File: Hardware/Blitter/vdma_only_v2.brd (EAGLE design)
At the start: 100 x 157.5 mm, 84 parts, among them IC1 74S08N, IC10 74HC191N, IC11 74HC191N, IC12 74HC191N, IC13 74HC191N, IC14 74HC191N, IC15 74HC191N, IC16 74HC573N, IC17 74HC573N, IC18 7432N, IC19 74LS257N, IC2 74HC191N, IC20 7430N, IC21 7400N, IC22 74LS257N, IC23 74LS257N, IC24 74LS257N, IC25 74LS257N, IC26 74LS257N, IC27 74LS257N, IC28 74LS257N, IC29 74LS257N, IC3 74HC573N, IC30 74HC573N, IC31 7400N, IC32 7432N, IC33 7400N, IC4 74HC191N, IC5 74HC573N, IC53 7404N, IC54 74LS07N, IC6 74HC573N, IC7 74HC573N, IC8 74HC573N, IC9 74LS74N, J1 TX25-40P-6ST-H1E, J2 TX25-40P-6ST-H1E

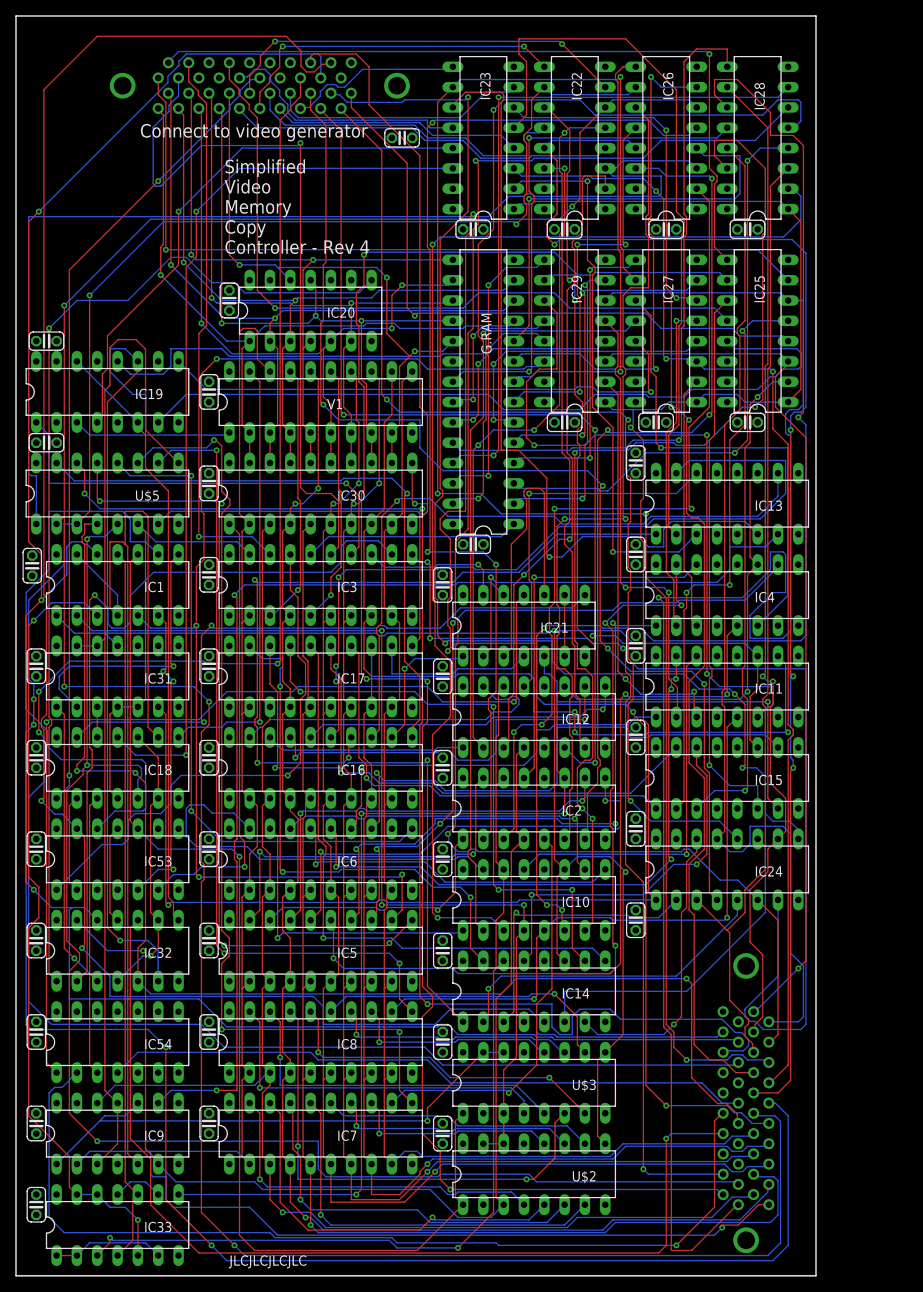
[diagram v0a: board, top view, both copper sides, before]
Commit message: regrettably I don't remember what I changed since the last commit
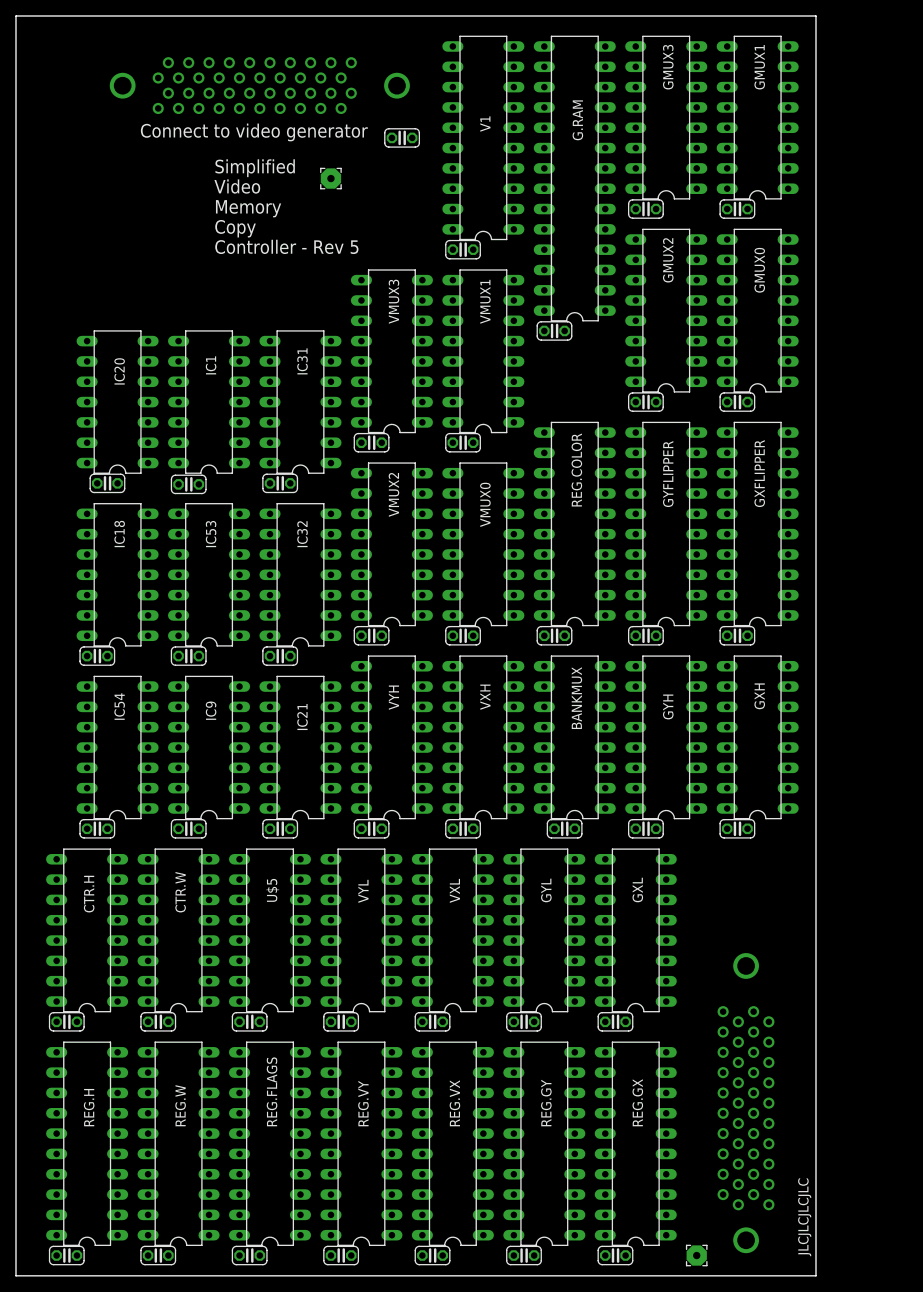
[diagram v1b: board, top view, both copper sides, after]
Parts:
- removed IC10, IC11, IC12, IC13, IC14, IC15, IC2, IC4: 74HC191N, 74xx-us:DIL16
- removed IC16, IC17, IC3, IC30, IC5, IC6, IC7, IC8: 74HC573N, 74xx-us:DIL20
- removed IC19, IC22, IC23, IC24, IC25, IC26, IC27, IC28, IC29: 74LS257N, 74xx-us:DIL16
- removed IC33: 7400N, 74xx-us:DIL14
- removed U$2, U$3: CD40103, 000_mychips2:DIL16
- added BANKMUX, GMUX0, GMUX1, GMUX2, GMUX3, VMUX0, VMUX1, VMUX2, VMUX3: 74LS257N, 74xx-us:DIL16
- added CTR.H, CTR.W: CD40103, 000_mychips2:DIL16
- added GXFLIPPER, GYFLIPPER: 74AHC8541, 0_gametankparts:DIL20
- added GXH, GXL, GYH, GYL, VXH, VXL, VYH, VYL: 74HC163, 0_gametankparts:DIL16
- added PAD1, PAD2: (no value), wirepad:2,54/0,9
- added REG.COLOR, REG.FLAGS, REG.GX, REG.GY, REG.H, REG.VX, REG.VY, REG.W: 74HC573N, 74xx-us:DIL20
- moved C5 114.9 mm to (63.5, 2.54), turned to 0 degrees
- moved C27 80.3 mm to (52.1, 2.54), turned to 0 degrees
- moved C8 79.6 mm to (90.2, 109.2), turned to 0 degrees
- moved C31 76.0 mm to (78.7, 55.9)
- moved C32 76.0 mm to (68.6, 55.9)
- moved C33 76.0 mm to (55.9, 55.9)
- moved C34 76.0 mm to (44.5, 55.9)
- moved C29 75.5 mm to (55.9, 128.3), turned to 0 degrees
- moved C28 74.5 mm to (40.6, 2.54), turned to 0 degrees
- moved C25 74.3 mm to (52.1, 31.8), turned to 0 degrees
- moved C9 71.8 mm to (74.9, 2.54), turned to 0 degrees
- moved C26 69.1 mm to (40.6, 31.8), turned to 0 degrees
- moved C21 63.8 mm to (78.7, 109.2), turned to 0 degrees
- moved C24 63.7 mm to (78.7, 133.3), turned to 0 degrees
- moved C36 59.7 mm to (90.2, 133.3), turned to 0 degrees
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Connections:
- removed net N$107: IC12.13, IC13.14
- removed net N$109: IC14.13, IC15.14
- removed net XCLK: IC10.14, IC12.14, IC14.14, IC2.14, IC33.3
- new net GX-CARRY: GXH.10, GXL.15
- new net GY-CARRY: GYH.10, GYL.15
- new net N$68: GXFLIPPER.7, GXH.13
- new net N$72: GXFLIPPER.8, GXH.12
- new net N$73: GYFLIPPER.2, GYL.14
- new net N$74: GYFLIPPER.3, GYL.13
- new net N$75: GYFLIPPER.4, GYL.12
- new net N$76: GYFLIPPER.5, GYL.11
- new net N$77: GYFLIPPER.6, GYH.14
- new net N$78: GYFLIPPER.7, GYH.13
- new net N$79: GYFLIPPER.8, GYH.12
- new net N$80: GYFLIPPER.1, IC53.4
- new net N$81: GXFLIPPER.1, IC31.8
- new net ROWCOMPLETE: GYL.10, IC53.8, VYL.10
- new net VX-CARRY: VXH.10, VXL.15
- new net VY-CARRY: VYH.10, VYL.15
- net !COPYDONE: now also CTR.H.14, CTR.H.15; no longer U$3.14, U$3.15
- net !DMA-ENABLED: now also CTR.W.3; no longer IC12.4, IC2.4, U$2.3
- net !DMACLK!/!IDLE!: now also CTR.H.1, CTR.W.1; no longer U$2.1, U$3.1
- net !DMAMODE: now also GMUX0.1, GMUX1.1, GMUX2.1, GMUX3.1, VMUX0.1, VMUX1.1, VMUX2.1, VMUX3.1; no longer IC22.1, IC23.1, IC24.1, IC25.1, IC26.1, IC27.1, IC28.1, IC29.1
- net !DMASTART: now also CTR.H.9, CTR.W.9, GYH.9, GYL.9, VYH.9, VYL.9; no longer IC10.11, IC11.11, IC14.11, IC15.11, U$2.9, U$3.9
- net !ROWCOMPLETE: now also CTR.H.3, CTR.W.14, CTR.W.15, IC53.9; no longer IC10.4, IC14.4, U$2.14, U$2.15, U$3.3
- net !VOE: now also VMUX3.12; no longer IC25.12
- net !VWE: now also VMUX1.12; no longer IC23.12
- net !WRAP_X: now also REG.VX.12; no longer IC16.12
- net !WRAP_Y: now also REG.VY.12; no longer IC17.12
- net !XRELOAD: now also GXH.9, GXL.9, IC1.3, VXH.9, VXL.9; no longer IC12.11, IC13.11, IC2.11, IC33.8, IC4.11
- net A0: now also GMUX0.3, VMUX0.3; no longer IC22.3, IC26.3
- net A1: now also GMUX0.6, VMUX0.6; no longer IC22.6, IC26.6
- net A10: now also GMUX2.13, VMUX2.13; no longer IC24.13, IC28.13
- net A11: now also GMUX3.3, VMUX3.3; no longer IC25.3, IC29.3
- net A12: now also GMUX3.6, VMUX3.6; no longer IC25.6, IC29.6
- net A13: now also GMUX3.10, VMUX3.10; no longer IC25.10, IC29.10
- net A2: now also GMUX0.10, VMUX0.10; no longer IC22.10, IC26.10
- net A3: now also GMUX0.13, VMUX0.13; no longer IC22.13, IC26.13
- net A4: now also GMUX1.3, VMUX1.3; no longer IC23.3, IC27.3
- net A5: now also GMUX1.6, VMUX1.6; no longer IC23.6, IC27.6
- net A6: now also GMUX1.10, VMUX1.10; no longer IC23.10, IC27.10
- net A7: now also GMUX2.3, VMUX2.3; no longer IC24.3, IC28.3
- net A8: now also GMUX2.6, VMUX2.6; no longer IC24.6, IC28.6
- net A9: now also GMUX2.10, VMUX2.10; no longer IC24.10, IC28.10
- net COLORFILL: now also GMUX3.14, REG.GX.12; no longer IC29.14, IC5.12
- net D0: now also REG.COLOR.2, REG.FLAGS.2, REG.GX.2, REG.GY.2, REG.H.2, REG.VX.2, REG.VY.2, REG.W.2; no longer IC16.2, IC17.2, IC3.2, IC30.2, IC5.2, IC6.2, IC7.2, IC8.2
- net D1: now also REG.COLOR.3, REG.FLAGS.3, REG.GX.3, REG.GY.3, REG.H.3, REG.VX.3, REG.VY.3, REG.W.3; no longer IC16.3, IC17.3, IC3.3, IC30.3, IC5.3, IC6.3, IC7.3, IC8.3
- net D2: now also REG.COLOR.4, REG.FLAGS.4, REG.GX.4, REG.GY.4, REG.H.4, REG.VX.4, REG.VY.4, REG.W.4; no longer IC16.4, IC17.4, IC3.4, IC30.4, IC5.4, IC6.4, IC7.4, IC8.4
- net D3: now also REG.COLOR.5, REG.FLAGS.5, REG.GX.5, REG.GY.5, REG.H.5, REG.VX.5, REG.VY.5, REG.W.5; no longer IC16.5, IC17.5, IC3.5, IC30.5, IC5.5, IC6.5, IC7.5, IC8.5
- net D4: now also REG.COLOR.6, REG.FLAGS.6, REG.GX.6, REG.GY.6, REG.H.6, REG.VX.6, REG.VY.6, REG.W.6; no longer IC16.6, IC17.6, IC3.6, IC30.6, IC5.6, IC6.6, IC7.6, IC8.6
- net D5: now also REG.COLOR.7, REG.FLAGS.7, REG.GX.7, REG.GY.7, REG.H.7, REG.VX.7, REG.VY.7, REG.W.7; no longer IC16.7, IC17.7, IC3.7, IC30.7, IC5.7, IC6.7, IC7.7, IC8.7
- net D6: now also REG.COLOR.8, REG.FLAGS.8, REG.GX.8, REG.GY.8, REG.H.8, REG.VX.8, REG.VY.8, REG.W.8; no longer IC16.8, IC17.8, IC3.8, IC30.8, IC5.8, IC6.8, IC7.8, IC8.8
- net D7: now also REG.COLOR.9, REG.FLAGS.9, REG.GX.9, REG.GY.9, REG.H.9, REG.VX.9, REG.VY.9, REG.W.9; no longer IC16.9, IC17.9, IC3.9, IC30.9, IC5.9, IC6.9, IC7.9, IC8.9
- net DD0: now also REG.COLOR.19; no longer IC30.19
- net DD1: now also REG.COLOR.18; no longer IC30.18
- net DD2: now also REG.COLOR.17; no longer IC30.17
- net DD3: now also REG.COLOR.16; no longer IC30.16
- net DD4: now also REG.COLOR.15; no longer IC30.15
- net DD5: now also REG.COLOR.14; no longer IC30.14
- net DD6: now also REG.COLOR.13; no longer IC30.13
- net DD7: now also REG.COLOR.12; no longer IC30.12
- net DMA-ENABLED: now also GXH.7, GXL.7, GYH.7, GYL.7, VXH.7, VXL.7, VYH.7, VYL.7; no longer IC1.13
- net DMACLK/!IDLE!: now also GXH.2, GXL.2, GYH.2, GYL.2, VXH.2, VXL.2, VYH.2, VYL.2; no longer IC33.10, IC33.4
- net DMAIRQEN: now also REG.FLAGS.13; no longer IC3.13
- net DMAMODE: now also REG.FLAGS.19; no longer IC3.19
- net GND: now also BANKMUX.15, BANKMUX.8, CTR.H.13, CTR.H.8, CTR.W.13, CTR.W.8, GMUX0.15, GMUX0.8, GMUX1.15, GMUX1.8, GMUX2.15, GMUX2.8, GMUX3.15, GMUX3.8, GXFLIPPER.10, GXFLIPPER.11, GXH.8, GXL.8, GYFLIPPER.10, GYFLIPPER.11, GYH.8, GYL.8, PAD1.1, PAD2.1, REG.COLOR.10, REG.FLAGS.1, REG.FLAGS.10, REG.GX.1, REG.GX.10, REG.GY.1, REG.GY.10, REG.H.1, REG.H.10, REG.VX.1, REG.VX.10, REG.VY.1, REG.VY.10, REG.W.1, REG.W.10, VMUX0.15, VMUX0.8, VMUX1.15, VMUX1.8, VMUX2.15, VMUX2.8, VMUX3.15, VMUX3.8, VXH.8, VXL.8, VYH.8, VYL.8; no longer IC10.8, IC11.4, IC11.8, IC11.9, IC12.5, IC12.8, IC13.4, IC13.5, IC13.8, IC13.9, IC14.5, IC14.8, IC15.4, IC15.5, IC15.8, IC15.9, IC16.1, IC16.10, IC17.1, IC17.10, IC19.15, IC19.8, IC2.8, IC22.15, IC22.8, IC23.15, IC23.8, IC24.15, IC24.8, IC25.15, IC25.8, IC26.15, IC26.8, IC27.15, IC27.8, IC28.15, IC28.8, IC29.15, IC29.8, IC3.1, IC3.10, IC30.10, IC31.10, IC31.9, IC33.7, IC4.4, IC4.8, IC4.9, IC5.1, IC5.10, IC53.3, IC53.9, IC6.1, IC6.10, IC7.1, IC7.10, IC8.1, IC8.10, U$2.13, U$2.8, U$3.13, U$3.8
- net GRAMBANK: now also REG.FLAGS.16; no longer IC3.16
- net N$1: now also GMUX0.4; no longer IC26.4
- net N$10: now also GMUX2.9; no longer IC28.9
- net N$108: now also REG.W.11; no longer IC7.11
- net N$11: now also GMUX2.12; no longer IC28.12
- net N$111: now also REG.H.11; no longer IC8.11
- net N$113: now also REG.VY.19, VYL.3; no longer IC14.15, IC17.19
- net N$114: now also REG.VY.18, VYL.4; no longer IC14.1, IC17.18
- net N$115: now also REG.VY.17, VYL.5; no longer IC14.10, IC17.17
- net N$116: now also REG.VY.16, VYL.6; no longer IC14.9, IC17.16
- net N$117: now also REG.VX.15, VXH.3; no longer IC13.15, IC16.15
- net N$118: now also REG.VX.14, VXH.4; no longer IC13.1, IC16.14
- net N$119: now also REG.VX.13, VXH.5; no longer IC13.10, IC16.13
- net N$12: now also GMUX3.4; no longer IC29.4
- net N$121: now also REG.VX.19, VXL.3; no longer IC12.15, IC16.19
- net N$122: now also REG.VX.18, VXL.4; no longer IC12.1, IC16.18
- net N$123: now also REG.VX.17, VXL.5; no longer IC12.10, IC16.17
- net N$124: now also REG.VX.16, VXL.6; no longer IC12.9, IC16.16
- net N$125: now also REG.COLOR.11; no longer IC30.11
- net N$13: now also GMUX3.7; no longer IC29.7
- net N$14: now also GMUX3.9; no longer IC29.9
- net N$15: now also VMUX1.14; no longer IC23.14
- net N$160: now also VMUX0.5, VXL.13; no longer IC12.2, IC22.5
- net N$161: now also VMUX0.11, VXL.12; no longer IC12.6, IC22.11
- net N$162: now also VMUX0.14, VXL.11; no longer IC12.7, IC22.14
- net N$163: now also VMUX1.2, VXH.14; no longer IC13.3, IC23.2
- net N$164: now also VMUX1.5, VXH.13; no longer IC13.2, IC23.5
- net N$165: now also VMUX1.11, VXH.12; no longer IC13.6, IC23.11
- net N$167: now also VMUX2.5, VYL.13; no longer IC14.2, IC24.5
- net N$168: now also VMUX2.11, VYL.12; no longer IC14.6, IC24.11
- net N$169: now also VMUX2.14, VYL.11; no longer IC14.7, IC24.14
- net N$17: now also GMUX1.12; no longer IC27.12
- net N$170: now also VMUX3.2, VYH.14; no longer IC15.3, IC25.2
- net N$171: now also VMUX3.5, VYH.13; no longer IC15.2, IC25.5
- net N$172: now also VMUX3.11, VYH.12; no longer IC15.6, IC25.11
- net N$173: now also GMUX0.2, GXFLIPPER.19; no longer IC2.3, IC26.2
- net N$174: now also GMUX0.5, GXFLIPPER.18; no longer IC2.2, IC26.5
- net N$175: now also GMUX0.11, GXFLIPPER.17; no longer IC2.6, IC26.11
- net N$176: now also GMUX0.14, GXFLIPPER.16; no longer IC2.7, IC26.14
- net N$177: now also GMUX1.2, GXFLIPPER.15; no longer IC27.2, IC4.3
- net N$178: now also GMUX1.5, GXFLIPPER.14; no longer IC27.5, IC4.2
- net N$179: now also GMUX1.11, GXFLIPPER.13; no longer IC27.11, IC4.6
- net N$18: now also GMUX3.12; no longer IC29.12
- net N$180: now also GMUX2.2, GYFLIPPER.19; no longer IC10.3, IC28.2
- net N$181: now also GMUX2.5, GYFLIPPER.18; no longer IC10.2, IC28.5
- net N$182: now also GMUX2.11, GYFLIPPER.17; no longer IC10.6, IC28.11
- net N$183: now also GMUX2.14, GYFLIPPER.16; no longer IC10.7, IC28.14
- net N$184: now also GMUX3.2, GYFLIPPER.15; no longer IC11.3, IC29.2
- net N$185: now also GMUX3.5, GYFLIPPER.14; no longer IC11.2, IC29.5
- net N$186: now also GMUX3.11, GYFLIPPER.13; no longer IC11.6, IC29.11
- net N$19: now also GYL.3, REG.GY.19; no longer IC10.15, IC6.19
- net N$2: now also GMUX0.7; no longer IC26.7
- net N$20: now also GYL.4, REG.GY.18; no longer IC10.1, IC6.18
- net N$21: now also GYL.5, REG.GY.17; no longer IC10.10, IC6.17
- net N$22: now also GYL.6, REG.GY.16; no longer IC10.9, IC6.16
- net N$23: now also GXH.3, REG.GX.15; no longer IC4.15, IC5.15
- net N$24: now also GXH.4, REG.GX.14; no longer IC4.1, IC5.14
- net N$25: now also GXH.5, REG.GX.13; no longer IC4.10, IC5.13
- net N$26: now also GYH.3, REG.GY.15; no longer IC11.15, IC6.15
- net N$27: now also GXL.3, REG.GX.19; no longer IC2.15, IC5.19
- net N$28: now also GXL.4, REG.GX.18; no longer IC2.1, IC5.18
- net N$29: now also GXL.5, REG.GX.17; no longer IC2.10, IC5.17
- net N$3: now also GMUX0.9; no longer IC26.9
- net N$30: now also GXL.6, REG.GX.16; no longer IC2.9, IC5.16
- net N$31: now also GYH.4, REG.GY.14; no longer IC11.1, IC6.14
- net N$32: now also GYH.5, REG.GY.13; no longer IC11.10, IC6.13
- net N$35: now also REG.VY.15, VYH.3; no longer IC15.15, IC17.15
- net N$36: now also REG.VY.14, VYH.4; no longer IC15.1, IC17.14
- net N$37: now also REG.VY.13, VYH.5; no longer IC15.10, IC17.13
- net N$4: now also GMUX0.12; no longer IC26.12
- net N$41: now also REG.COLOR.1; no longer IC30.1
- net N$42: now also GXFLIPPER.5, GXL.11; no longer IC2.13, IC4.14
- net N$43: now also GXFLIPPER.4, GXL.12; no longer IC10.13, IC11.14
- net N$47: now also GXFLIPPER.3, GXL.13; no longer IC1.3, IC33.12, IC33.13, IC33.5
- net N$48: now also GXFLIPPER.2, GXL.14; no longer IC33.11, IC33.9
- net N$49: now also GXFLIPPER.6, GXH.14; no longer IC33.1, IC33.2, IC33.6
- net N$5: now also GMUX1.4; no longer IC27.4
- net N$50: now also BANKMUX.4, VMUX1.13; no longer IC19.4, IC23.13
- net N$51: now also CTR.H.4, REG.H.19; no longer IC8.19, U$3.4
- net N$52: now also CTR.H.5, REG.H.18; no longer IC8.18, U$3.5
- net N$53: now also CTR.H.6, REG.H.17; no longer IC8.17, U$3.6
- net N$54: now also CTR.H.7, REG.H.16; no longer IC8.16, U$3.7
- net N$55: now also CTR.H.10, REG.H.15; no longer IC8.15, U$3.10
- net N$56: now also CTR.H.11, REG.H.14; no longer IC8.14, U$3.11
- net N$57: now also CTR.H.12, REG.H.13; no longer IC8.13, U$3.12
- net N$59: now also CTR.W.4, REG.W.19; no longer IC7.19, U$2.4
- net N$6: now also GMUX1.7; no longer IC27.7
- net N$60: now also CTR.W.5, REG.W.18; no longer IC7.18, U$2.5
- net N$61: now also CTR.W.6, REG.W.17; no longer IC7.17, U$2.6
- net N$62: now also CTR.W.7, REG.W.16; no longer IC7.16, U$2.7
- net N$63: now also CTR.W.10, REG.W.15; no longer IC7.15, U$2.10
- net N$64: now also CTR.W.11, REG.W.14; no longer IC7.14, U$2.11
- net N$65: now also CTR.W.12, REG.W.13; no longer IC7.13, U$2.12
- net N$67: now also BANKMUX.7, VMUX3.13; no longer IC19.7, IC25.13
- net N$69: now also BANKMUX.9, GMUX1.13; no longer IC19.9, IC27.13
- net N$7: now also GMUX1.9; no longer IC27.9
- net N$70: now also BANKMUX.12, GMUX3.13; no longer IC19.12, IC29.13
- net N$71: now also REG.VX.11; no longer IC16.11
- net N$8: now also GMUX2.4; no longer IC28.4
- net N$9: now also GMUX2.7; no longer IC28.7
- net N$94: now also REG.VY.11; no longer IC17.11
- net N$96: now also REG.GX.11; no longer IC5.11
- net N$98: now also REG.GY.11; no longer IC6.11
- net OFFSCR_X: now also VXH.11; no longer IC13.7
- net OFFSCR_Y: now also VYH.11; no longer IC15.7
- net TRANSEN: now also REG.FLAGS.12; no longer IC3.12
- net V/_G: now also BANKMUX.1, REG.FLAGS.14; no longer IC19.1, IC3.14
- net VA0: now also VMUX0.4; no longer IC22.4
- net VA1: now also VMUX0.7; no longer IC22.7
- net VA10: now also VMUX2.12; no longer IC24.12
- net VA11: now also VMUX3.4; no longer IC25.4
- net VA12: now also VMUX3.7; no longer IC25.7
- net VA13: now also VMUX3.9; no longer IC25.9
- net VA2: now also VMUX0.9; no longer IC22.9
- net VA3: now also VMUX0.12; no longer IC22.12
- net VA4: now also VMUX1.4; no longer IC23.4
- net VA5: now also VMUX1.7; no longer IC23.7
- net VA6: now also VMUX1.9; no longer IC23.9
- net VA7: now also VMUX2.4; no longer IC24.4
- net VA8: now also VMUX2.7; no longer IC24.7
- net VA9: now also VMUX2.9; no longer IC24.9
- net VCC: now also BANKMUX.10, BANKMUX.13, BANKMUX.16, BANKMUX.2, BANKMUX.5, CTR.H.16, CTR.H.2, CTR.W.16, CTR.W.2, GMUX0.16, GMUX1.14, GMUX1.16, GMUX2.16, GMUX3.16, GXFLIPPER.20, GXH.1, GXH.16, GXL.1, GXL.10, GXL.16, GYFLIPPER.20, GYH.1, GYH.16, GYL.1, GYL.16, IC1.13, REG.COLOR.20, REG.FLAGS.20, REG.GX.20, REG.GY.20, REG.H.20, REG.VX.20, REG.VY.20, REG.W.20, VMUX0.16, VMUX1.16, VMUX2.16, VMUX3.14, VMUX3.16, VXH.1, VXH.16, VXL.1, VXL.10, VXL.16, VYH.1, VYH.16, VYL.1, VYL.16; no longer IC10.16, IC11.16, IC12.16, IC13.16, IC14.16, IC15.16, IC16.20, IC17.20, IC19.10, IC19.13, IC19.16, IC19.2, IC19.5, IC2.16, IC22.16, IC23.16, IC24.16, IC25.14, IC25.16, IC26.16, IC27.14, IC27.16, IC28.16, IC29.16, IC3.20, IC30.20, IC33.14, IC4.16, IC5.20, IC6.20, IC7.20, IC8.20, U$2.16, U$2.2, U$3.16, U$3.2
- net VG_OE: now also BANKMUX.14, BANKMUX.6; no longer IC19.14, IC19.6
- net VG_WE: now also BANKMUX.11, BANKMUX.3; no longer IC19.11, IC19.3
- net VIDFLAGS: now also REG.FLAGS.11; no longer IC3.11
- net VIDPAGE: now also REG.FLAGS.18; no longer IC3.18
- net VNMI_ENABLE: now also REG.FLAGS.17; no longer IC3.17
- net VRAMBANK: now also REG.FLAGS.15; no longer IC3.15
- net XDIR: now also IC31.10, IC31.9, REG.W.12; no longer IC2.5, IC4.5, IC7.12
- net XODD: now also VMUX0.2, VXL.14; no longer IC12.3, IC22.2
- net YDIR: now also IC53.3, REG.H.12; no longer IC10.5, IC11.5, IC8.12
- net YODD: now also VMUX2.2, VYL.14; no longer IC14.3, IC24.2
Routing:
- net A2: track 323.2 -> 0.00 mm, vias 6 -> 0
- net A0: track 295.7 -> 0.00 mm, vias 4 -> 0
- net CLK14: track 254.0 -> 0.00 mm, vias 3 -> 0
- net CLK28: track 243.6 -> 0.00 mm, vias 2 -> 0
- net CLK3_5: track 237.9 -> 0.00 mm, vias 3 -> 0
- net D0: track 229.6 -> 0.00 mm, vias 1 -> 0
- net !DMAMODE: track 237.6 -> 14.6 mm, vias 2 -> 0
- net A1: track 321.5 -> 104.4 mm, vias 5 -> 0
- net A13: track 214.2 -> 0.00 mm, vias 4 -> 0
- net D1: track 210.1 -> 0.00 mm, vias 2 -> 0
- net A6: track 207.7 -> 0.00 mm, vias 4 -> 0
- net A12: track 200.2 -> 0.00 mm, vias 1 -> 0
- net VA8: track 196.3 -> 0.00 mm, vias 3 -> 0
- net D3: track 195.3 -> 0.00 mm, vias 2 -> 0
- net !DMASTART: track 192.2 -> 0.00 mm, vias 2 -> 0
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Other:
- board text added: "Designed by Clyde Shaffer January 2021"
- board text added: "Simplified Video Memory Copy Controller - Rev 5"
- board text removed: "Designed by Clyde Shaffer December 2020"
- board text removed: "Simplified Video Memory Copy Controller - Rev 4"

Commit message: Blitter V6 w/ 4-phase clock
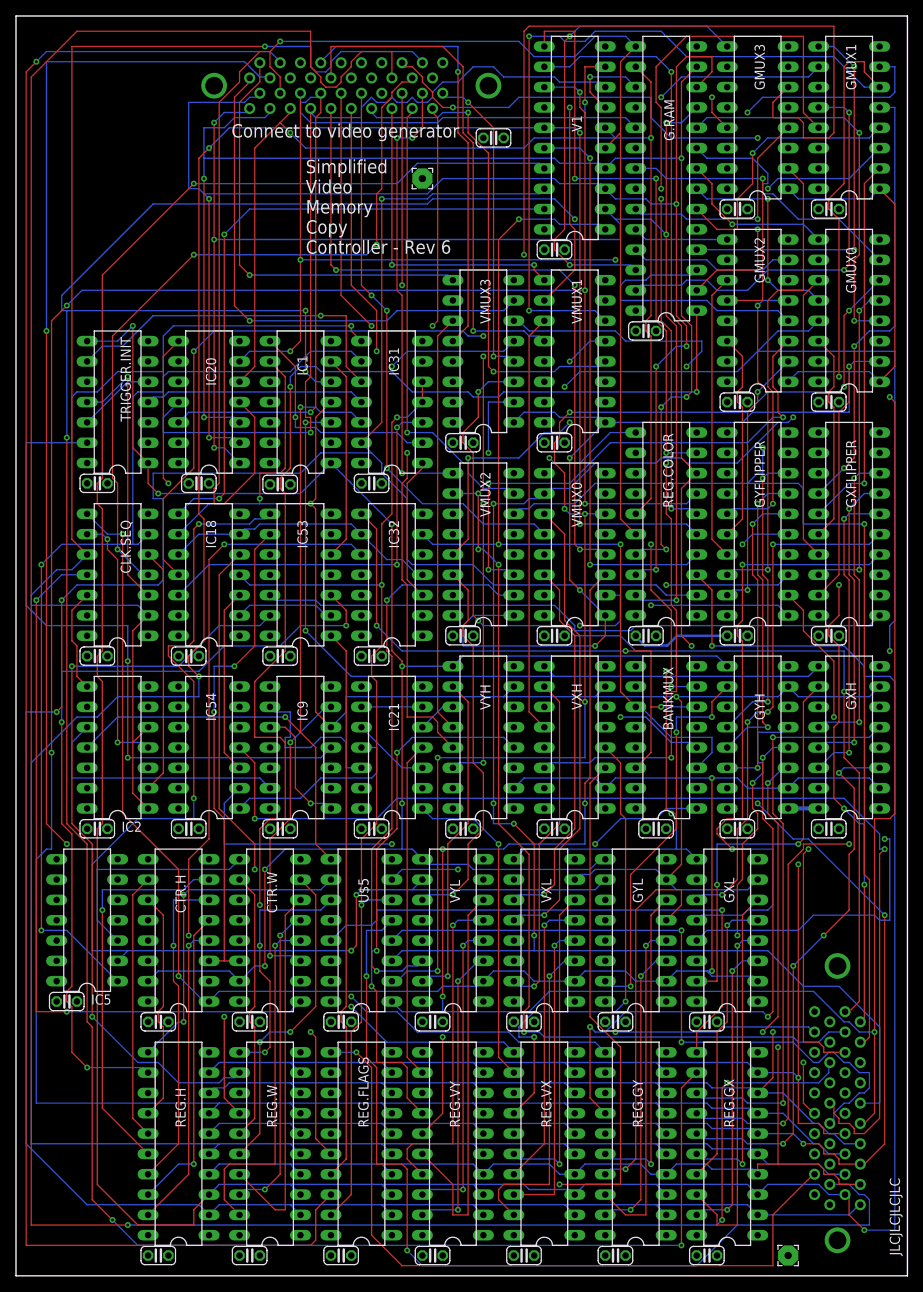
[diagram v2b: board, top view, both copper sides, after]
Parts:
- added C42, C43, C44, C46: (no value), rcl:C025-024X044
- added CLK.SEQ: 74ALS08N, 74xx-us:DIL14
- added IC2: 74ALS04N, 74xx-us:DIL14
- added IC5: 74ALS00N, 74xx-us:DIL14
- added TRIGGER.INIT: 74LS74N, 74xx-us:DIL14
- moved BANKMUX 11.4 mm to (81.3, 67.3)
- moved C21 11.4 mm to (90.2, 109.2)
- moved C22 11.4 mm to (74.9, 31.8)
- moved C24 11.4 mm to (90.2, 133.3)
- moved C31 11.4 mm to (90.2, 55.9)
- moved C32 11.4 mm to (80.0, 55.9)
- moved C40 11.4 mm to (90.2, 80.0)
- moved C5 11.4 mm to (74.9, 2.54)
- moved G.RAM 11.4 mm to (81.3, 137.2)
- moved GMUX0 11.4 mm to (104.1, 120.7)
- moved GMUX1 11.4 mm to (104.1, 144.8)
- moved GXFLIPPER 11.4 mm to (104.1, 94.0)
- moved GXH 11.4 mm to (104.1, 67.3)
- moved GXL 11.4 mm to (88.9, 43.2)
- moved J1 11.4 mm to (106.7, 21.6)
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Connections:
- net !DMAIRQ renamed !IRQ-OUT
- net DMAIRQEN renamed IRQ-ENABLE
- net N$58 renamed IRQ
- removed net !CLK28: IC1.9, IC53.12
- removed net !DMA-ENABLED: CTR.W.3, IC32.13, IC9.6
- removed net !DMACLK!/!IDLE!: CTR.H.1, CTR.W.1, IC1.10, IC53.10
- removed net !DMASTART: CTR.H.9, CTR.W.9, GYH.9, GYL.9, IC1.1, IC31.11, VYH.9, VYL.9
- removed net DMA-ENABLED: GXH.7, GXL.7, GYH.7, GYL.7, IC1.4, IC18.9, IC9.5, VXH.7, VXL.7, VYH.7, VYL.7
- removed net DMACLK/!IDLE!: GXH.2, GXL.2, GYH.2, GYL.2, IC1.11, VXH.2, VXL.2, VYH.2, VYL.2
- removed net DMACLK/IDLE: IC32.11, IC53.11
- removed net DMASTART: IC31.12, IC31.13, IC9.11, IC9.3, U$5.9
- new net !INIT: CTR.H.15, CTR.W.15, GYH.9, GYL.9, IC1.1, TRIGGER.INIT.1, TRIGGER.INIT.8, VYH.9, VYL.9
- new net !RUNNING: CTR.W.3, IC9.6
- new net !TRIGGER: IC31.11, TRIGGER.INIT.4
- new net N$58: IC31.10, TRIGGER.INIT.9
- new net N$82: IC31.8, IC9.4, TRIGGER.INIT.13
- new net N$83: CLK.SEQ.13, IC2.6
- new net N$84: CLK.SEQ.12, IC2.8
- new net N$85: CLK.SEQ.5, IC2.2
- new net N$86: CLK.SEQ.9, IC2.4
- new net N$87: CTR.W.9, IC5.3
- new net N$88: IC2.10, IC9.13
- new net P0: CLK.SEQ.11, CTR.W.1
- new net P1: CLK.SEQ.8, CTR.H.1, GXH.2, GXL.2, GYH.2, GYL.2, VXH.2, VXL.2, VYH.2, VYL.2
- new net P2: CLK.SEQ.6, IC31.9, IC5.1
- new net P3: CLK.SEQ.3, IC1.10, TRIGGER.INIT.11
- new net RUNNING: GXH.7, GXL.7, GYH.7, GYL.7, IC1.4, IC1.9, IC18.9, IC9.5, VXH.7, VXL.7, VYH.7, VYL.7
- new net TRIGGER-FLAG: TRIGGER.INIT.12, TRIGGER.INIT.5
- new net TRIGGER-SELECT: IC2.11, IC31.12, U$5.9
- net !COPYDONE: no longer CTR.H.15
- net !ROWCOMPLETE: no longer CTR.W.15
- net CLK14: now also CLK.SEQ.1, CLK.SEQ.4, IC2.3, IC2.9; no longer IC1.12, IC32.12
- net CLK28: now also CLK.SEQ.10, CLK.SEQ.2, IC2.1, IC2.5; no longer IC53.13
- net D0: now also IC31.13; no longer IC9.2
- net D1: no longer IC9.12
- net GND: now also C42.2, C43.2, C44.2, C46.2, CLK.SEQ.7, IC2.7, IC5.7, IC9.11, IC9.12, IC9.2, IC9.3, TRIGGER.INIT.2, TRIGGER.INIT.3, TRIGGER.INIT.7
- net N$81: now also IC53.12; no longer IC31.8
- net ROWCOMPLETE: now also IC5.2
- net VCC: now also C42.1, C43.1, C44.1, C46.1, CLK.SEQ.14, CTR.H.9, IC2.14, IC5.14, TRIGGER.INIT.10, TRIGGER.INIT.14; no longer IC1.13, IC9.13, IC9.4
- net XDIR: now also IC53.13; no longer IC31.10, IC31.9
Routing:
- net D1: track 0.00 -> 398.1 mm, vias 0 -> 3
- net D3: track 0.00 -> 368.5 mm, vias 0 -> 4
- net D0: track 0.00 -> 354.6 mm, vias 0 -> 3
- net COLORFILL: track 0.00 -> 347.8 mm, vias 0 -> 6
- net CLK3_5: track 0.00 -> 321.4 mm, vias 0 -> 3
- net D5: track 46.3 -> 352.6 mm, vias 0 -> 5
- net CLK28: track 0.00 -> 262.3 mm, vias 0 -> 2
- net D4: track 0.00 -> 253.1 mm, vias 0 -> 5
- net D6: track 0.00 -> 248.0 mm, vias 0 -> 3
- net A12: track 0.00 -> 247.2 mm, vias 0 -> 2
- net D2: track 0.00 -> 245.4 mm, vias 0 -> 3
- net A0: track 0.00 -> 239.6 mm, vias 0 -> 5
- net D7: track 16.2 -> 253.8 mm, vias 0 -> 5
- net CLK14: track 0.00 -> 228.6 mm, vias 0 -> 3
- net VIDPAGE: track 0.00 -> 223.1 mm, vias 0 -> 1
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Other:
- board size 100 x 157.5 mm -> 111.4 x 157.5 mm
- board text added: "Designed by Clyde Shaffer April 2021"
- board text added: "Simplified Video Memory Copy Controller - Rev 6"
- board text removed: "Designed by Clyde Shaffer January 2021"
- board text removed: "Simplified Video Memory Copy Controller - Rev 5"
